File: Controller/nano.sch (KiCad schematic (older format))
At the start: 24 parts, among them J10 ICSP, K1 SW_RESET, U2 INTERFACE-CH340T_SSOP20_, U3 MCU-ATMEGA328P-AU_TQFP32_, Y1 12MHz, Y2 16MHZ

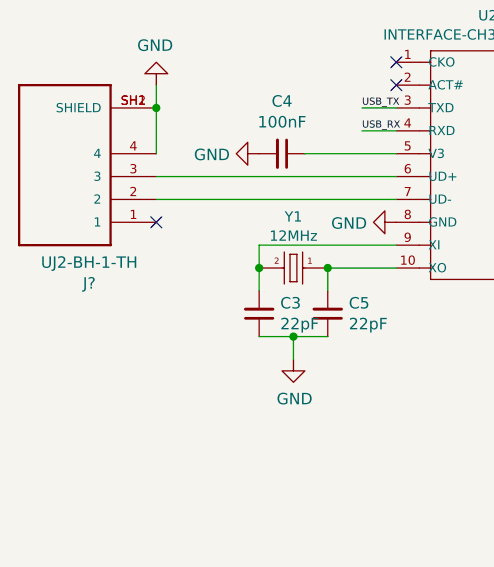
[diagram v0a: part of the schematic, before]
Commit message: More power routing
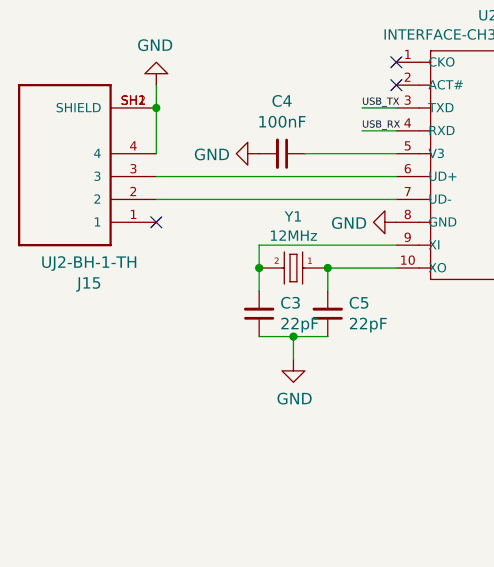
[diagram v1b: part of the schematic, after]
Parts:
- gave numbers to parts that had none: 1
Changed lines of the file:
@@
 Connection ~ 6800 1400
 $Comp
-L UJ2-BH-1-TH:UJ2-BH-1-TH J?
+L UJ2-BH-1-TH:UJ2-BH-1-TH J15
 U 1 1 5D55598E
 P 3300 2150
-F 0 "J?" H 3407 2617 50  0000 C CNN
+F 0 "J15" H 3407 2617 50  0000 C CNN
 F 1 "UJ2-BH-1-TH" H 3407 2526 50  0000 C CNN
 F 2 "CUI:CUI_UJ2-BH-1-TH" H 3300 2150 50  0001 L BNN
